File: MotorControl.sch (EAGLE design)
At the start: 47 parts

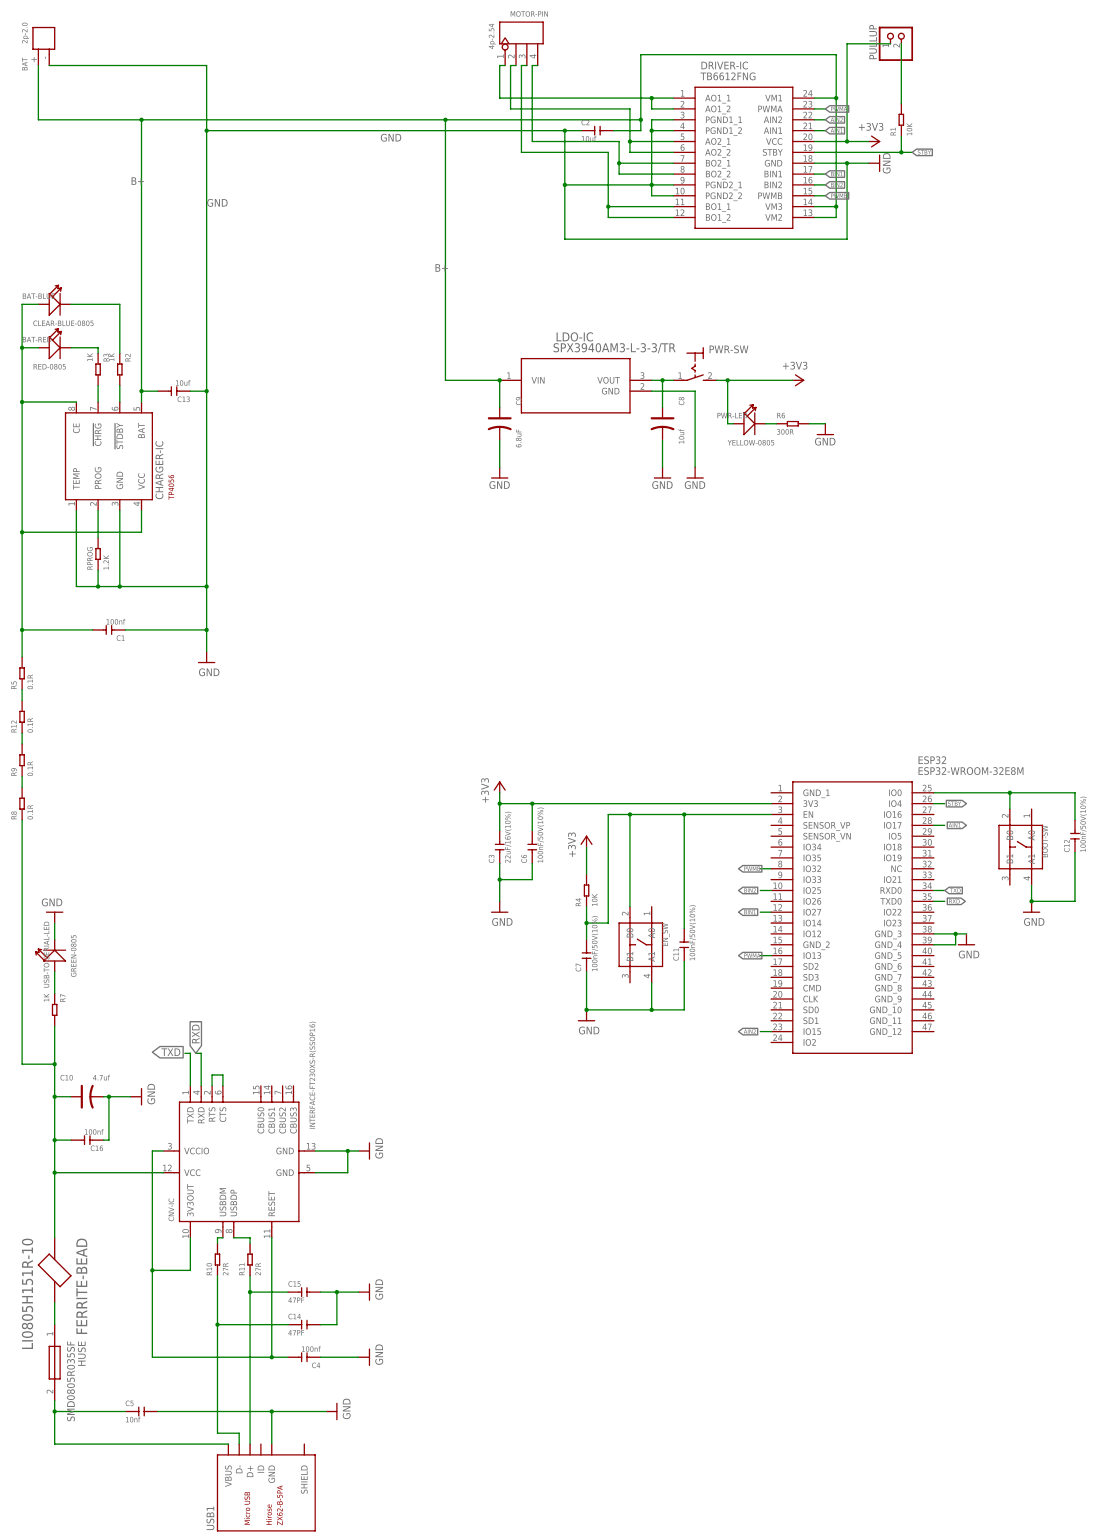
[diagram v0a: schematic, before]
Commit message: [Fix] 20210920MT時点（４層）
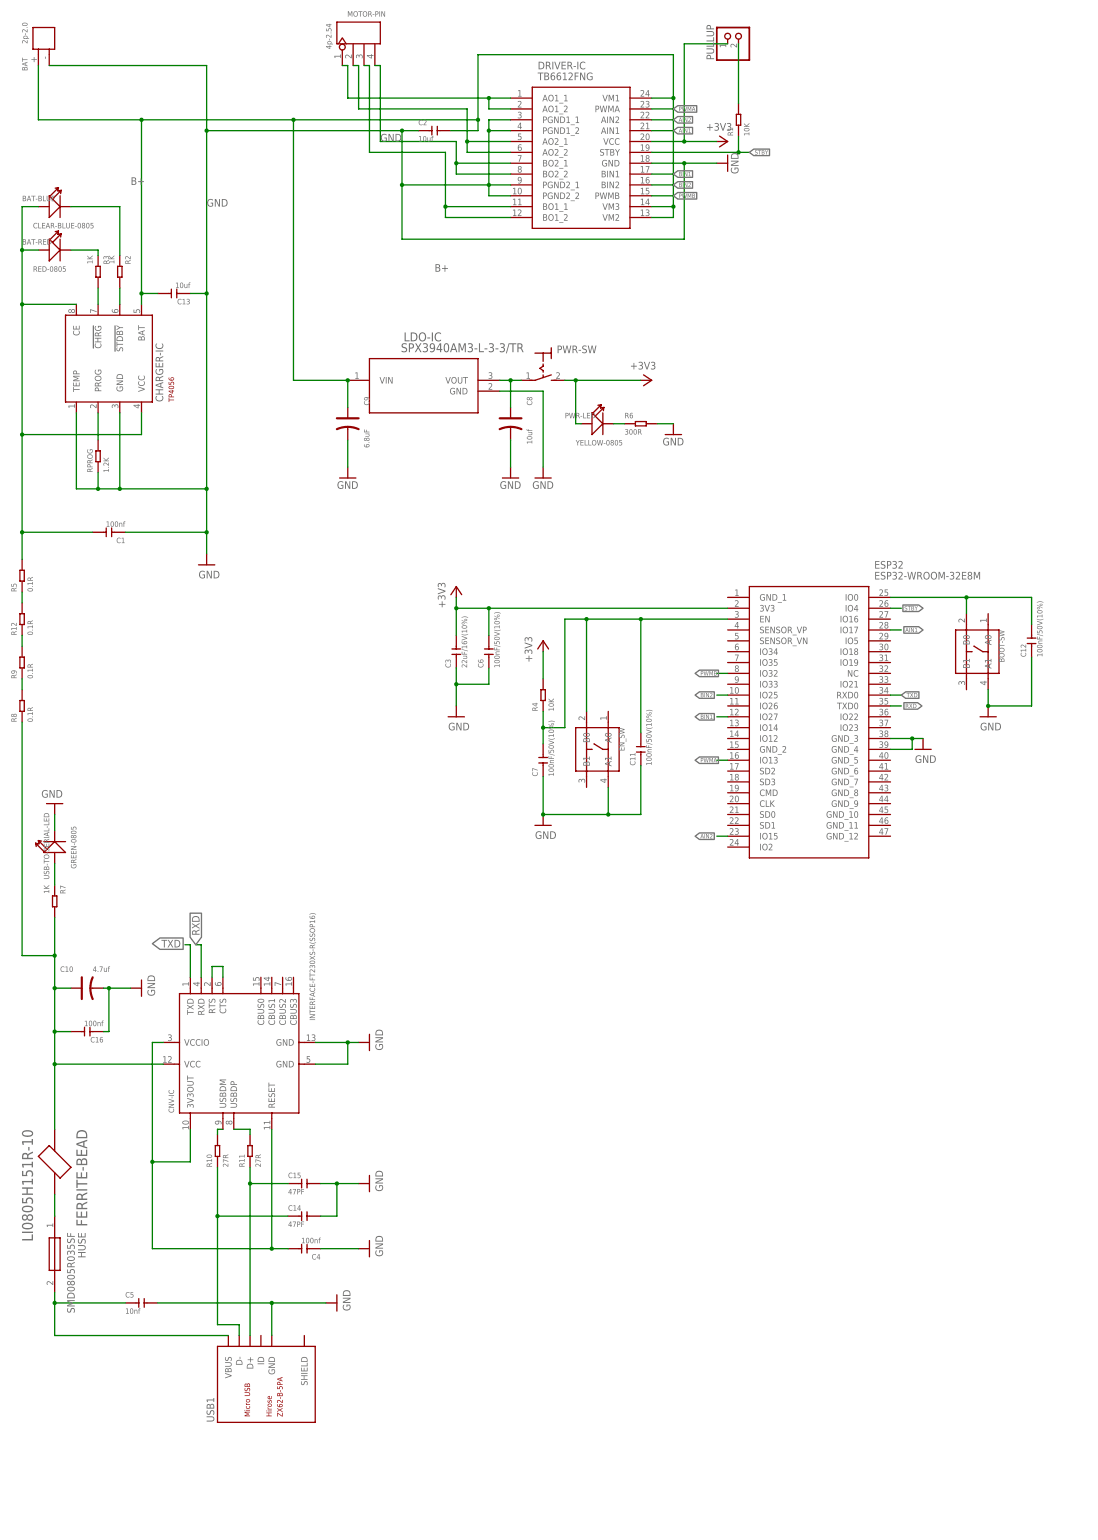
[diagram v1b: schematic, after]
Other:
- moved on the sheet: BAT-BLUE, BAT-RED, BOOT-SW, C1, C10, C11, C12, C13, C14, C15, C16, C2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
